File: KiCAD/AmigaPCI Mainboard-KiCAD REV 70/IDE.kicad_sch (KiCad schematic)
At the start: 57 parts, among them CN900 PRIMARY IDE, CN901 SECONDARY IDE, Q900 MMBT3906, U220 74LVC08, U815 74LVC08, U900 74LVC245, U901 74LVC245, U902 74LVC245, U903 74LVC245, U904 74LVC245, U905 74LVC245, U906 74LVC373, U907 74LVC373

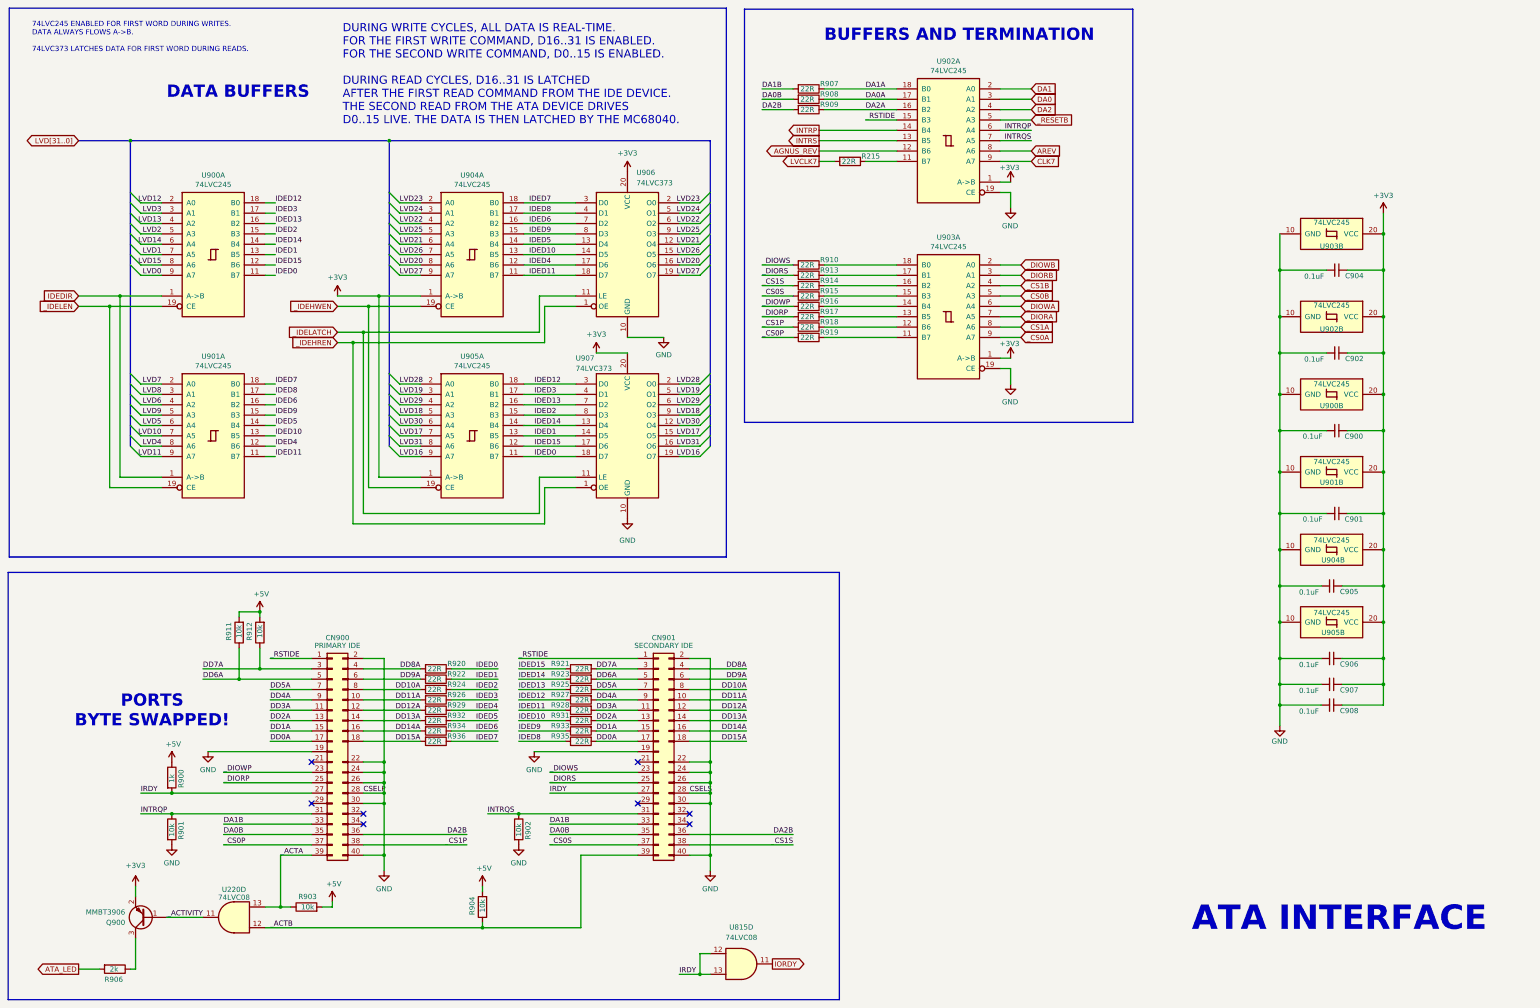
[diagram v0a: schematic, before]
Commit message: AmigaPCI Revision 7.0
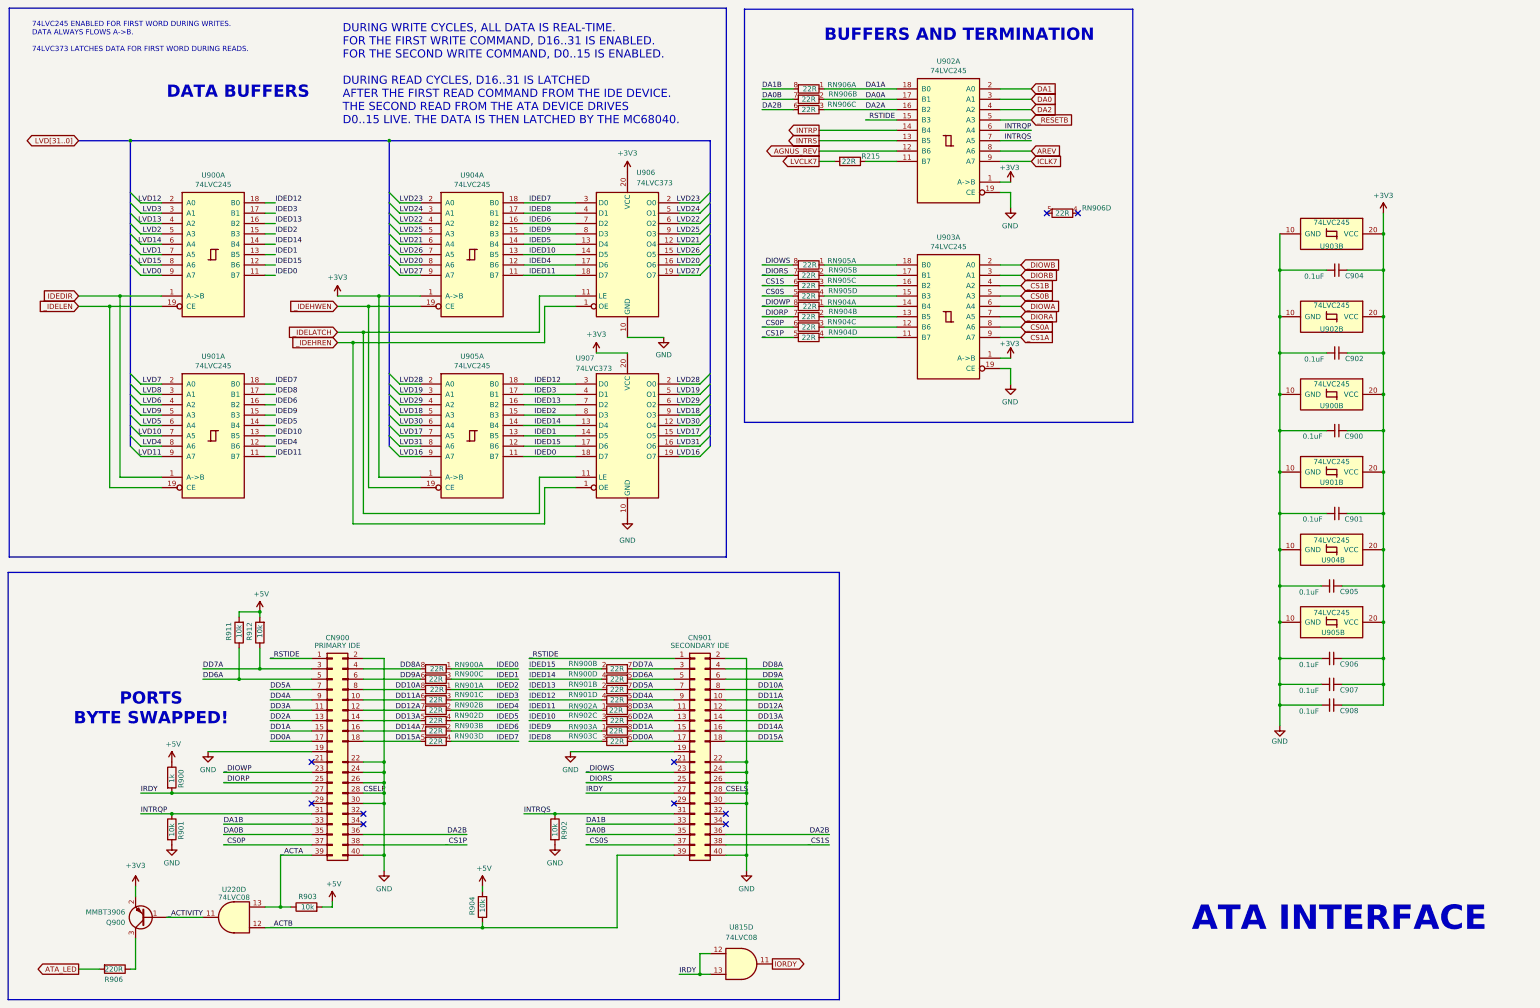
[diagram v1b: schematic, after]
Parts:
- removed R907, R908, R909, R910, R913, R914, R915, R916, R917, R918, R919, R920, R921, R922, R923, R924, R925, R926, R927, R928, R929, R931, R932, R933, R934, R935, R936: 22R, Resistor_SMD:R_0603_1608Metric, symbol Device:R
- added RN900, RN901, RN902, RN903, RN904, RN905, RN906: 22R, Resistor_SMD:R_Array_Convex_4x0603, symbol Device:R_Pack04_Split
- R906: value 2k -> 220R
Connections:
- net DA0A: now also RN906.2 (R2.1)
- net DA0B: now also RN906.7 (R2.2)
- net DA1A: now also RN906.1 (R1.1)
- net DA1B: now also RN906.8 (R1.2)
- net DA2A: now also RN906.3 (R3.1)
- net DA2B: now also RN906.6 (R3.2)
- net DD0A: now also RN903.6 (R3.2)
- net DD10A: now also RN901.8 (R1.2)
- net DD11A: now also RN901.6 (R3.2)
- net DD12A: now also RN902.7 (R2.2)
- net DD13A: now also RN902.5 (R4.2)
- net DD14A: now also RN903.7 (R2.2)
- net DD15A: now also RN903.5 (R4.2)
- net DD1A: now also RN903.8 (R1.2)
- net DD2A: now also RN902.6 (R3.2)
- net DD3A: now also RN902.8 (R1.2)
- net DD4A: now also RN901.5 (R4.2)
- net DD5A: now also RN901.7 (R2.2)
- net DD6A: now also RN900.5 (R4.2)
- net DD7A: now also RN900.7 (R2.2)
- net DD8A: now also RN900.8 (R1.2)
- net DD9A: now also RN900.6 (R3.2)
- net IDED0: now also RN900.1 (R1.1)
- net IDED1: now also RN900.3 (R3.1)
- net IDED10: now also RN902.3 (R3.1)
- net IDED11: now also RN902.1 (R1.1)
- net IDED12: now also RN901.4 (R4.1)
- net IDED13: now also RN901.2 (R2.1)
- net IDED14: now also RN900.4 (R4.1)
- net IDED15: now also RN900.2 (R2.1)
- net IDED2: now also RN901.1 (R1.1)
- net IDED3: now also RN901.3 (R3.1)
- net IDED4: now also RN902.2 (R2.1)
- net IDED5: now also RN902.4 (R4.1)
- net IDED6: now also RN903.2 (R2.1)
- net IDED7: now also RN903.4 (R4.1)
- net IDED8: now also RN903.3 (R3.1)
- net IDED9: now also RN903.1 (R1.1)
- net _CS0A: now also U903.8 (A6); no longer U903.9 (A7)
- net _CS0P: now also RN904.6 (R3.2)
- net _CS0S: now also RN905.5 (R4.2)
- net _CS1A: now also U903.9 (A7); no longer U903.8 (A6)
- net _CS1P: now also RN904.5 (R4.2)
- net _CS1S: now also RN905.6 (R3.2)
- net _DIORP: now also RN904.7 (R2.2)
- net _DIORS: now also RN905.7 (R2.2)
- net _DIOWP: now also RN904.8 (R1.2)
- net _DIOWS: now also RN905.8 (R1.2)
- net at U903.18 (B0): now also RN905.1 (R1.1)
- net at U903.16 (B2): now also RN905.3 (R3.1)
- net at U903.17 (B1): now also RN905.2 (R2.1)
- net at U903.13 (B5): now also RN904.2 (R2.1)
- net at U903.14 (B4): now also RN904.1 (R1.1)
- net at U903.11 (B7): now also RN904.4 (R4.1)
- net at U903.12 (B6): now also RN904.3 (R3.1)
- net at U903.15 (B3): now also RN905.4 (R4.1)
- net CLK7 renamed ICLK7
- no-connect marks 8 -> 10
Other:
- moved on the sheet: CN901, R902
